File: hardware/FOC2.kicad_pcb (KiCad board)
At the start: 4 copper layers, 40 x 40 mm, 98 parts, among them J1 Conn_01x03, J3 复用Typec, J4 Conn_01x02, J6 Conn_01x04, J7 Conn_01x03, Q1 Q_NMOS_SGD, Q2 Q_NMOS_SGD, Q3 Q_NMOS_SGD, Q4 Q_NMOS_SGD, Q5 Q_NMOS_SGD, Q6 Q_NMOS_SGD, U1 LM321, U10 REF3033, U2 CH340N, U3 STM32G431CBUx, U4 EG2133, U5 INA199xxDCK, U6 INA199xxDCK, U7 TPS54360DDA, U8 TJA1044GTK/3Z, U9 LP5907MFX-3.3

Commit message: 工程重构
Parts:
- C10, C11, C12, C13, C14, C15, C16, C17, C9: footprint Capacitor_SMD:C_1812_4532Metric -> FOCLibrary:C_1812_4532Metric
- C18, C19, C20, C21, C22, C23, C24, C25, C26, C27, C28, C29, C30, C31, C32, C33, C34, C35, C36, C37, C38, C39, C4, C5, C6, C7, C8: footprint Capacitor_SMD:C_0603_1608Metric -> FOCLibrary:C_0603_1608Metric
- D1, D3: footprint Diode_SMD:D_SMA -> FOCLibrary:D_SMA
- D10, D11, D2: footprint Diode_SMD:D_SOD-323_HandSoldering -> FOCLibrary:D_SOD-323_HandSoldering
- D12: footprint Diode_SMD:Nexperia_CFP3_SOD-123W -> FOCLibrary:Nexperia_CFP3_SOD-123W
- D13: footprint LED_SMD:LED_0603_1608Metric -> FOCLibrary:LED_0603_1608Metric
- D4, D5, D6, D7, D8, D9: footprint Diode_SMD:D_SOD-123 -> FOCLibrary:D_SOD-123
- H1, H2, H3, H4: footprint MountingHole:MountingHole_2.2mm_M2_DIN965_Pad -> FOCLibrary:MountingHole_2.2mm_M2_DIN965_Pad
- J1: footprint Connector_AMASS:AMASS_MR30PW-FB_1x03_P3.50mm_Horizontal -> FOCLibrary:AMASS_MR30PW-FB_1x03_P3.50mm_Horizontal
- J3: footprint Connector_USB:USB_C_Receptacle_HRO_TYPE-C-31-M-12 -> FOCLibrary:USB_C_Receptacle_HRO_TYPE-C-31-M-12
- J4: footprint Connector_AMASS:AMASS_XT30PW-F_1x02_P2.50mm_Horizontal -> FOCLibrary:AMASS_XT30PW-F_1x02_P2.50mm_Horizontal
- J6: footprint Connector_Molex:Molex_PicoBlade_53047-0410_1x04_P1.25mm_Vertical -> FOCLibrary:Molex_PicoBlade_53047-0410_1x04_P1.25mm_Vertical
- J7: footprint Connector_Molex:Molex_PicoBlade_53047-0310_1x03_P1.25mm_Vertical -> FOCLibrary:Molex_PicoBlade_53047-0310_1x03_P1.25mm_Vertical
- L1: footprint Inductor_SMD:L_Abracon_ASPI-0630LR -> FOCLibrary:L_Abracon_ASPI-0630LR
- Q1, Q2, Q3, Q4, Q5, Q6: footprint Package_SON:VSONP-8-1EP_5x6_P1.27mm -> FOCLibrary:VSONP-8-1EP_5x6_P1.27mm
- R1, R10, R11, R12, R13, R14, R15, R16, R17, R18, R19, R2, R23, R24, R25, R26, R4, R5, R7, R8: footprint Resistor_SMD:R_0603_1608Metric -> FOCLibrary:R_0603_1608Metric
- R3, R6, R9: footprint Resistor_SMD:R_2512_6332Metric -> FOCLibrary:R_2512_6332Metric
- U1, U9: footprint Package_TO_SOT_SMD:SOT-23-5 -> FOCLibrary:SOT-23-5
- U10: footprint Package_TO_SOT_SMD:SOT-23 -> FOCLibrary:SOT-23
- U2: footprint Package_SO:SOP-8_3.9x4.9mm_P1.27mm -> FOCLibrary:SOP-8_3.9x4.9mm_P1.27mm
- U3: footprint Package_DFN_QFN:QFN-48-1EP_7x7mm_P0.5mm_EP5.6x5.6mm -> FOCLibrary:QFN-48-1EP_7x7mm_P0.5mm_EP5.6x5.6mm
- U4: footprint Package_SO:TSSOP-20_4.4x6.5mm_P0.65mm -> FOCLibrary:TSSOP-20_4.4x6.5mm_P0.65mm
- U5, U6: footprint Package_TO_SOT_SMD:SOT-363_SC-70-6 -> FOCLibrary:SOT-363_SC-70-6
- U7: footprint Package_SO:TI_SO-PowerPAD-8_ThermalVias -> FOCLibrary:TI_SO-PowerPAD-8_ThermalVias
- U8: footprint Package_SON:HVSON-8-1EP_3x3mm_P0.65mm_EP1.6x2.4mm -> FOCLibrary:HVSON-8-1EP_3x3mm_P0.65mm_EP1.6x2.4mm

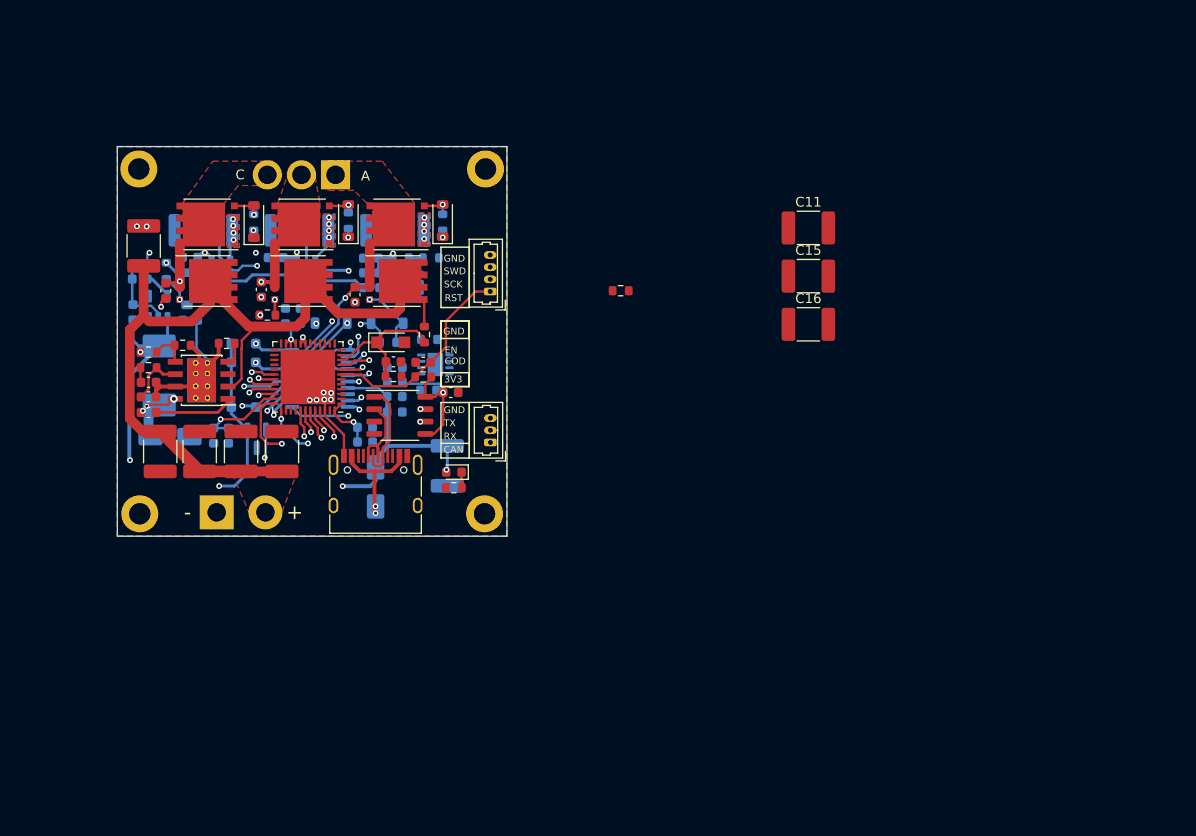
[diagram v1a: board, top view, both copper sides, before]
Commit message: 添加驱动设计
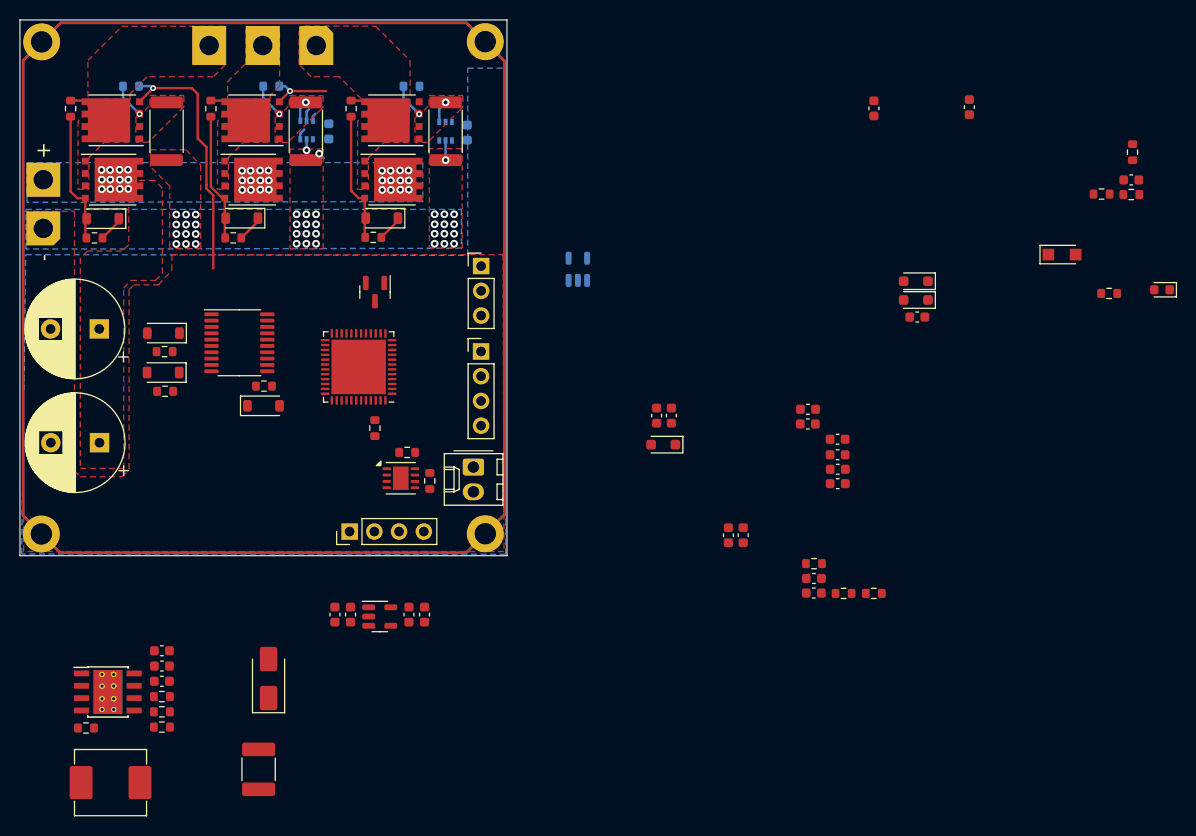
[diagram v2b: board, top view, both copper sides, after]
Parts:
- removed C10, C11, C12, C13, C14, C15, C9: 47uf, FOCLibrary:C_1812_4532Metric
- removed C30: 10uf, FOCLibrary:C_0603_1608Metric
- removed C4: 100nf, FOCLibrary:C_0603_1608Metric
- removed D1: type="D" model="ss34" lib="", FOCLibrary:D_SMA
- removed J3: 复用Typec, FOCLibrary:USB_C_Receptacle_HRO_TYPE-C-31-M-12
- removed J7: Conn_01x03, FOCLibrary:Molex_PicoBlade_53047-0310_1x03_P1.25mm_Vertical
- removed U2: CH340N, FOCLibrary:SOP-8_3.9x4.9mm_P1.27mm
- added C1: 470uf, Capacitor_THT:CP_Radial_D10.0mm_P5.00mm, F.Cu at (30.2, 170.4)
- added J2: Conn_01x02, Connector_Molex:Molex_KK-254_AE-6410-02A_1x02_P2.54mm_Vertical, F.Cu at (68.6, 172.9)
- added J8: Conn_01x03, Connector_PinHeader_2.54mm:PinHeader_1x03_P2.54mm_Vertical, F.Cu at (69.3, 152.3)
- added J9: Conn_01x04, Connector_PinHeader_2.54mm:PinHeader_1x04_P2.54mm_Vertical, F.Cu at (69.3, 161.0)
- added R20: 10k, Resistor_SMD:R_0603_1608Metric, F.Cu at (58.4, 168.9)
- added R21: 120, Resistor_SMD:R_0603_1608Metric, F.Cu at (64.1, 174.3)
- added R22: 10k, Resistor_SMD:R_0603_1608Metric, F.Cu at (41.6, 136.1)
- added R27: 10k, Resistor_SMD:R_0603_1608Metric, F.Cu at (56.0, 136.1)
- added R28: 10k, Resistor_SMD:R_0603_1608Metric, B.Cu at (62.2, 133.8)
- added R29: 10k, Resistor_SMD:R_0603_1608Metric, B.Cu at (47.8, 133.8)
- C16: value 47uf -> 470uf; footprint FOCLibrary:C_1812_4532Metric -> Capacitor_THT:CP_Radial_D10.0mm_P5.00mm
- C17: footprint FOCLibrary:C_1812_4532Metric -> Library:C_1812_4532Metric; moved to F.Cu
- C18, C19, C20, C23, C24, C25, C28, C29, C33: footprint FOCLibrary:C_0603_1608Metric -> Library:C_0603_1608Metric
- C21, C22, C26, C27, C31, C32, C34, C35, C36, C37, C38, C39, C5, C6, C7, C8: footprint FOCLibrary:C_0603_1608Metric -> Library:C_0603_1608Metric; moved to F.Cu
- D10, D11, D2: footprint FOCLibrary:D_SOD-323_HandSoldering -> Library:D_SOD-323_HandSoldering; moved to F.Cu
- D12: footprint FOCLibrary:Nexperia_CFP3_SOD-123W -> Library:Nexperia_CFP3_SOD-123W
- D13: footprint FOCLibrary:LED_0603_1608Metric -> Library:LED_0603_1608Metric
- D3: footprint FOCLibrary:D_SMA -> Library:D_SMA; moved to F.Cu
- D4, D6, D8: footprint FOCLibrary:D_SOD-123 -> Library:D_SOD-123; moved to F.Cu
- D5, D7, D9: footprint FOCLibrary:D_SOD-123 -> Library:D_SOD-123
- H1, H2, H3, H4: footprint FOCLibrary:MountingHole_2.2mm_M2_DIN965_Pad -> Library:MountingHole_2.2mm_M2_DIN965_Pad
- J1: footprint FOCLibrary:AMASS_MR30PW-FB_1x03_P3.50mm_Horizontal -> Library:AMASS_MR30PW-FB_1x03_P3.50mm_Horizontal
- J4: footprint FOCLibrary:AMASS_XT30PW-F_1x02_P2.50mm_Horizontal -> Library:AMASS_XT30PW-F_1x02_P2.50mm_Horizontal; moved to B.Cu
- J6: footprint FOCLibrary:Molex_PicoBlade_53047-0410_1x04_P1.25mm_Vertical -> Connector_PinHeader_2.54mm:PinHeader_1x04_P2.54mm_Vertical
- L1: footprint FOCLibrary:L_Abracon_ASPI-0630LR -> Library:L_Abracon_ASPI-0630LR; moved to F.Cu
- Q1, Q2, Q3, Q4, Q5, Q6: footprint FOCLibrary:VSONP-8-1EP_5x6_P1.27mm -> Library:VSONP-8-1EP_5x6_P1.27mm
- R1, R13, R14, R19, R2, R5, R7, R8: footprint FOCLibrary:R_0603_1608Metric -> Library:R_0603_1608Metric; moved to F.Cu
- R10: value 0 -> 10k; footprint FOCLibrary:R_0603_1608Metric -> Resistor_SMD:R_0603_1608Metric; moved to F.Cu
- R11: value 0 -> 10k; footprint FOCLibrary:R_0603_1608Metric -> Resistor_SMD:R_0603_1608Metric
- R12, R15, R16, R17, R18, R23, R24, R25, R26, R4: footprint FOCLibrary:R_0603_1608Metric -> Library:R_0603_1608Metric
- R3, R6, R9: value 0.0005 -> 0.001; footprint FOCLibrary:R_2512_6332Metric -> Library:R_2512_6332Metric; moved to F.Cu
- U1: footprint FOCLibrary:SOT-23-5 -> Library:SOT-23-5
- U10: footprint FOCLibrary:SOT-23 -> Library:SOT-23; moved to F.Cu
- U3: footprint FOCLibrary:QFN-48-1EP_7x7mm_P0.5mm_EP5.6x5.6mm -> Library:QFN-48-1EP_7x7mm_P0.5mm_EP5.6x5.6mm
- U4: footprint FOCLibrary:TSSOP-20_4.4x6.5mm_P0.65mm -> Library:TSSOP-20_4.4x6.5mm_P0.65mm; moved to F.Cu
- U5, U6: footprint FOCLibrary:SOT-363_SC-70-6 -> Library:SOT-363_SC-70-6
- U7: footprint FOCLibrary:TI_SO-PowerPAD-8_ThermalVias -> Library:TI_SO-PowerPAD-8_ThermalVias
- U8: footprint FOCLibrary:HVSON-8-1EP_3x3mm_P0.65mm_EP1.6x2.4mm -> Library:HVSON-8-1EP_3x3mm_P0.65mm_EP1.6x2.4mm; moved to F.Cu
- U9: footprint FOCLibrary:SOT-23-5 -> Library:SOT-23-5; moved to F.Cu
- moved D13 75.1 mm to (139.2, 154.7)
- moved R23 75.1 mm to (133.1, 144.9)
- moved C23 75.1 mm to (119.5, 135.9)
- moved C25 75.1 mm to (109.7, 136.1)
- moved R24 75.1 mm to (136.2, 140.6)
- moved C33 75.1 mm to (136.1, 143.4)
- moved R25 75.1 mm to (136.1, 144.9)
- moved C16 72.8 mm to (30.1, 158.7), turned to 180 degrees
- moved R26 70.2 mm to (133.8, 155.1)
- moved D2 69.5 mm to (114.0, 153.8)
- moved D12 69.5 mm to (129.0, 151.1)
- moved D11 69.2 mm to (114.0, 155.8)
- moved C24 57.8 mm to (114.1, 157.5), turned to 180 degrees
- moved R13 57.1 mm to (106.6, 185.9)
- moved R14 57.1 mm to (109.7, 185.9)
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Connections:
- H1 pad 1: GND -> Earth
- H2 pad 1: GND -> Earth
- H3 pad 1: GND -> Earth
- H4 pad 1: GND -> Earth
- R10 pad 1: /FDCAN_TX -> Net-(D4-A)
- R10 pad 2: Net-(U8-TXD) -> /VS1
- R11 pad 1: /FDCAN_RX -> Net-(D5-A)
- R11 pad 2: Net-(U8-RXD) -> /M1_SL_A
- U3 pad 19: /VREF -> unconnected-(U3-PB2-Pad19)
- U3 pad 41: /EN1 -> unconnected-(U3-PB3-Pad41)
- U3 pad 42: /EN2 -> unconnected-(U3-PB4-Pad42)
- U3 pad 43: /EN3 -> unconnected-(U3-PB5-Pad43)
- U3 pad 46: GND -> Net-(U3-PB8)
- U8 pad 1: Net-(U8-TXD) -> /FDCAN_TX
- U8 pad 4: Net-(U8-RXD) -> /FDCAN_RX
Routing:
- net Earth: track 0.00 -> 397.2 mm
- net +3.3V: track 137.2 -> 1.18 mm, vias 9 -> 0
- net +5V: track 94.1 -> 0.00 mm, vias 5 -> 0
- net VDC: track 83.7 -> 0.00 mm, vias 0 -> 36
- net /SWDIO: track 45.0 -> 0.00 mm, vias 1 -> 0
- net GND: track 45.3 -> 5.45 mm, vias 8 -> 39
- net /FDCAN_TX: track 39.3 -> 0.00 mm, vias 1 -> 0
- net /SWCLK: track 39.1 -> 0.00 mm, vias 2 -> 0
- net /M1_GL_A: track 30.2 -> 0.00 mm, vias 2 -> 0
- net /M1_GL_C: track 30.0 -> 0.00 mm, vias 2 -> 0
- net /FDCAN_RX: track 29.5 -> 0.00 mm, vias 1 -> 0
- net /M1_GH_C: track 28.7 -> 2.68 mm, vias 2 -> 0
- net /HIN_2: track 25.8 -> 0.00 mm, vias 3 -> 0
- net /VS3: track 29.9 -> 4.70 mm, vias 2 -> 0
- net Net-(D5-A): track 2.75 -> 27.2 mm
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- added copper zone on B.Cu, net VDC
- removed copper zone on B.Cu, net /M1_SL_A
- removed copper zone on B.Cu, net /M1_SL_B
- removed copper zone on B.Cu, net /M1_SL_C
- removed copper zone on In1.Cu, net GND
- removed copper zone on In2.Cu, net GND
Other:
- board size 40 x 40 mm -> 50 x 55 mm
- copper layers 4 -> 2
- board text removed: "3V3"
- board text removed: "A"
- board text removed: "C"
- board text removed: "CAN"
- board text removed: "DesignedBy ZhuYiping"
- board text removed: "EN COD"
- board text removed: "GND"
- board text removed: "RST"
- board text removed: "RX"
- board text removed: "SCK"
- board text removed: "SWD"
- board text removed: "TX"
